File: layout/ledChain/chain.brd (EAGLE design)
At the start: 28.1 x 15.7 mm, 26 parts, among them IC2 FT232RL, IC4 ATTINY85-20S, Q1 25mhz, T1 BC848, T2 BC848, U1 SPX3819M5-L-3-3

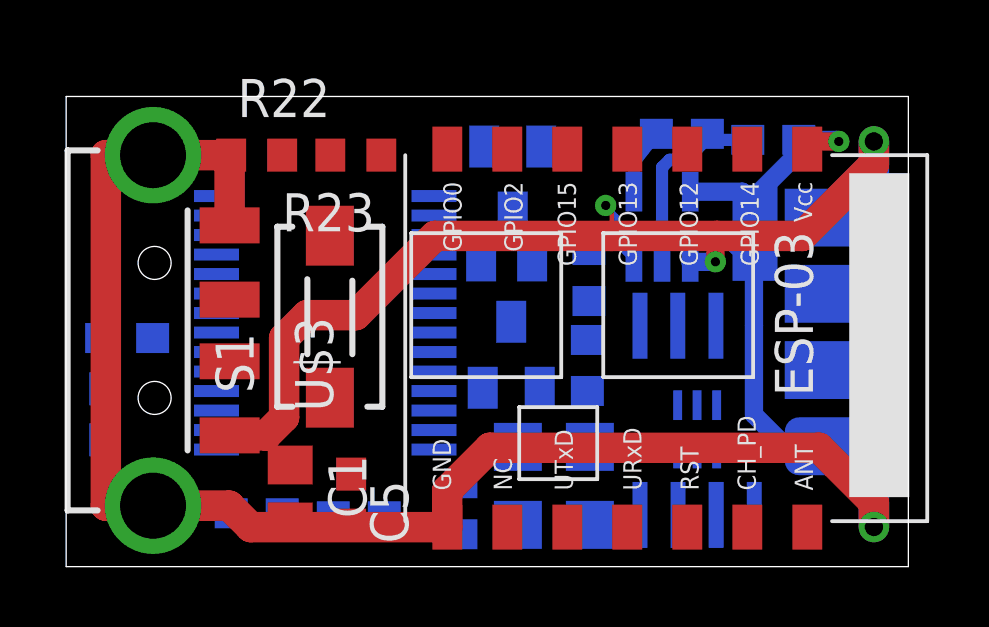
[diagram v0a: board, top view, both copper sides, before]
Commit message: challenge accepted and passed
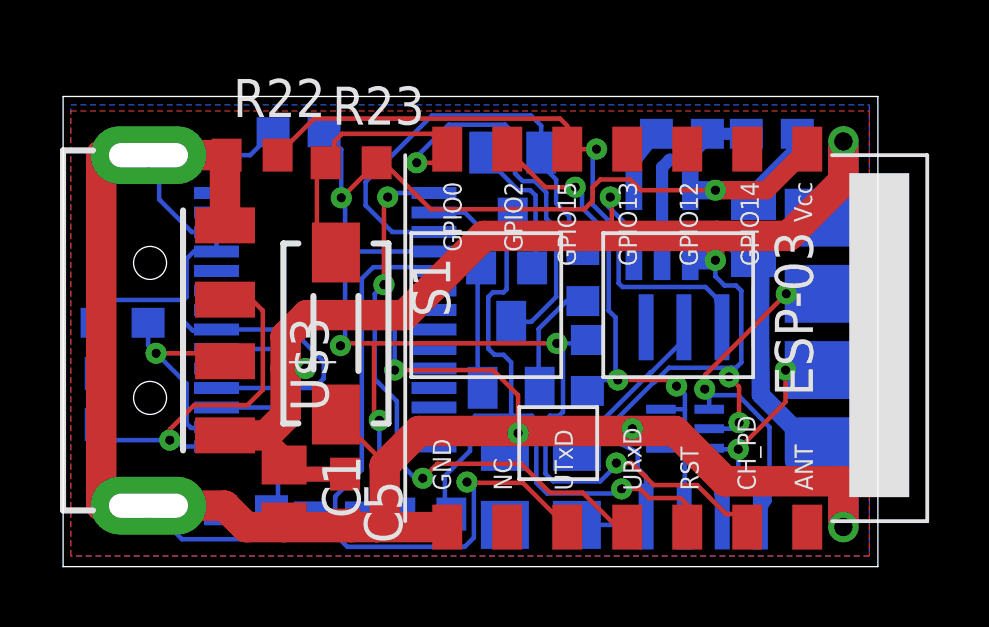
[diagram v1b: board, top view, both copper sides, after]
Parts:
- added C10: 100n, rcl:C0603
- moved R20 1.18 mm to (61.0, 49.8), turned to 0 degrees
- moved C9 0.76 mm to (58.0, 49.7)
- moved S1 0.59 mm to (58.0, 55.8), turned to 270 degrees
- moved C3 0.53 mm to (50.9, 56.1)
- moved C4 0.53 mm to (50.1, 53.6)
- moved Q1 0.43 mm to (64.8, 50.7)
- moved U$1 0.41 mm to (69.6, 52.6), turned to 90 degrees
- moved C2 0.37 mm to (55.0, 49.9)
- moved R23 0.30 mm to (58.5, 61.5), turned to 0 degrees
- moved C7 0.21 mm to (72.5, 62.4)
- moved IC4 0.21 mm to (70.3, 52.8)
- moved C1 0.20 mm to (56.3, 50.4)
- moved C5 0.20 mm to (58.3, 50.2)
- moved R3 0.20 mm to (66.2, 57.7)
- moved T1 0.20 mm to (63.9, 60.7)
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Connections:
- net +3V3: now also C10.1, IC2.4
- net GND: now also C10.2
- net N$15: no longer IC2.4
- net WSCLK: now also U$1.4; no longer U$1.6
- net WSDATA: now also U$1.6; no longer U$1.4
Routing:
- net +3V3: track 7.60 -> 60.7 mm, vias 1 -> 6
- net GND: track 70.1 -> 122.9 mm, vias 1 -> 4
- net RST: track 0.00 -> 25.5 mm, vias 0 -> 1
- net +5V: track 36.2 -> 60.8 mm, vias 3 -> 6
- net TX: track 0.00 -> 22.4 mm, vias 0 -> 1
- net GPIO0: track 0.00 -> 21.7 mm, vias 0 -> 1
- net GPIO15: track 0.00 -> 21.3 mm, vias 0 -> 1
- net RX: track 0.00 -> 19.9 mm, vias 0 -> 3
- net GPIO2: track 0.00 -> 19.1 mm, vias 0 -> 3
- net N$1: track 0.00 -> 15.1 mm
- net WSCLK: track 0.00 -> 12.6 mm, vias 0 -> 2
- net N$3: track 0.00 -> 12.2 mm, vias 0 -> 1
- net WSDATA: track 0.00 -> 8.73 mm, vias 0 -> 2
- net N$5: track 0.00 -> 7.54 mm
- net N$4: track 0.00 -> 7.36 mm, vias 0 -> 1
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- added copper zone on layer 1, net GND
- added copper zone on layer 16, net GND
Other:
- board size 28.1 x 15.7 mm -> 27.2 x 15.7 mm
